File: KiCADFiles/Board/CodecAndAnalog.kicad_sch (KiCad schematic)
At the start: 38 parts, among them J1 XLR, J2 MONO JACK, J4 MONO JACK, J5 MONO JACK, J6 MONO JACK, J7 MONO JACK, K2 Fujitsu_FTR-LYCA005x, U5 CS4272, U9 OPA1655D, X1 24.576 MHz 20 pF

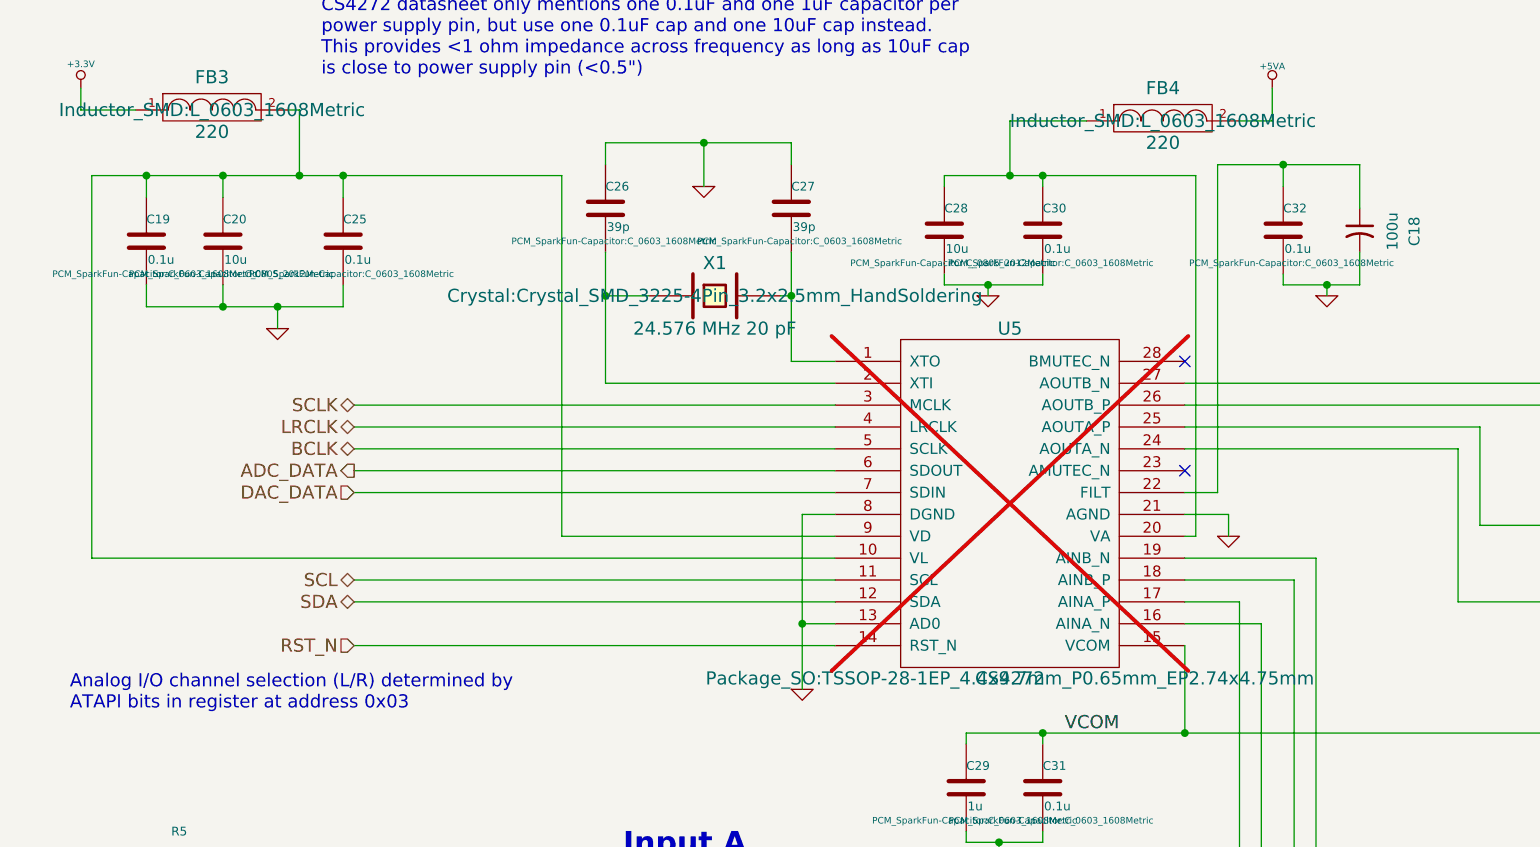
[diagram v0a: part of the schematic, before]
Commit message: improved layout further
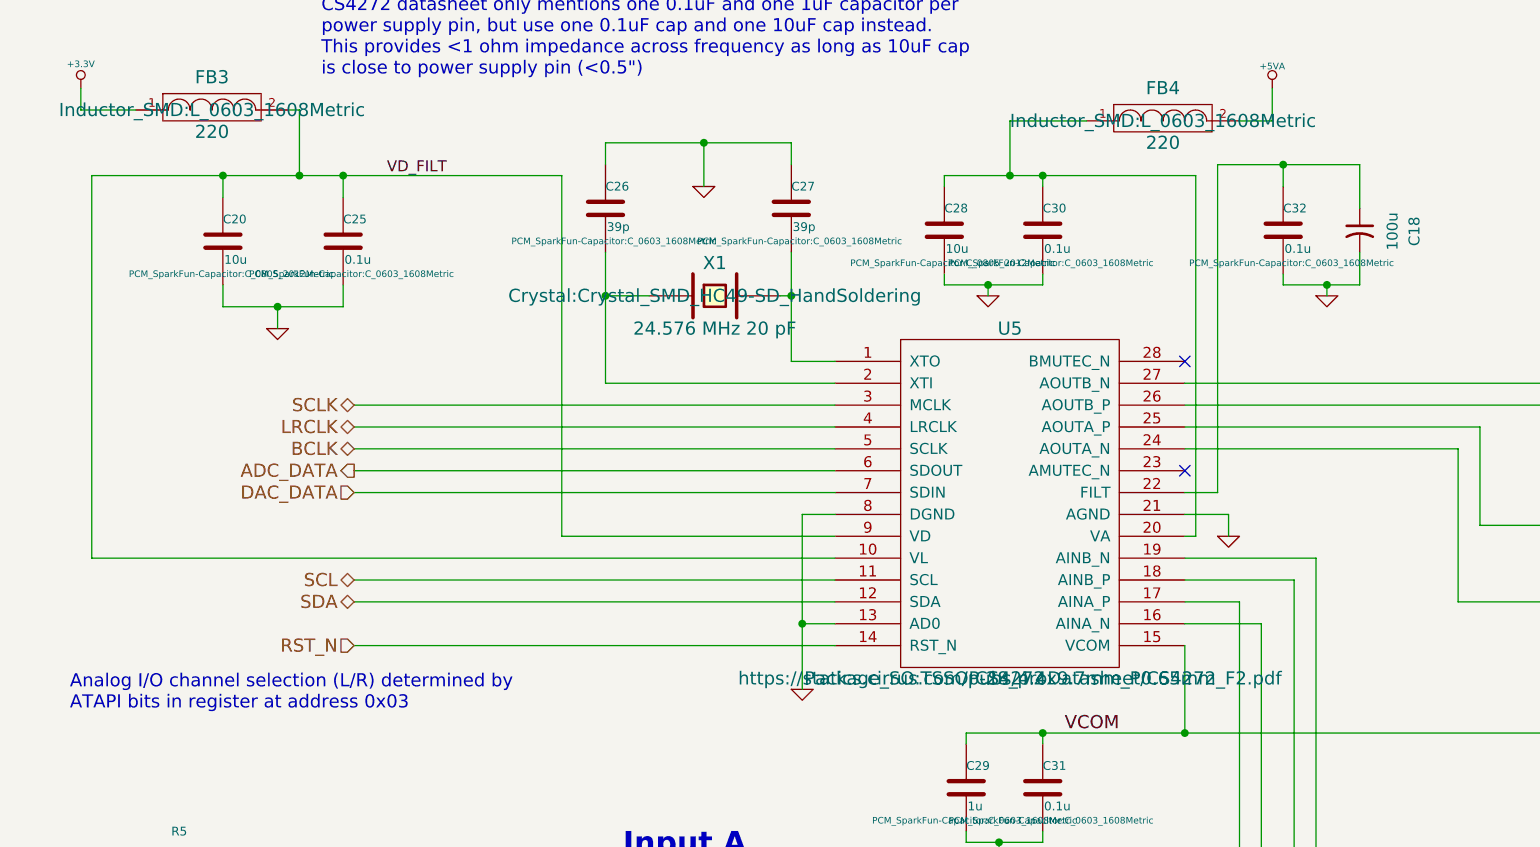
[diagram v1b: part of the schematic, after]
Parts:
- removed C19: 0.1u, PCM_SparkFun-Capacitor:C_0603_1608Metric, symbol SuperAudioBoard-rescue:C
- U5: footprint Package_SO:TSSOP-28-1EP_4.4x9.7mm_P0.65mm_EP2.74x4.75mm -> Package_SO:TSSOP-28_4.4x9.7mm_P0.65mm; now fitted
- X1: footprint Crystal:Crystal_SMD_3225-4Pin_3.2x2.5mm_HandSoldering -> Crystal:Crystal_SMD_HC49-SD_HandSoldering
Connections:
- net VD_FILT: now reaches C20.1, C25.1, FB3.2, U5.10 (VL), U5.9 (VD)
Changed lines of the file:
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@@
 	)
 	(junction
-		(at 25.4 29.21)
-		(diameter 0)
-		(color 0 0 0 0)
-	)
-	(junction
 		(at 129.54 93.98)
 		(diameter 0)
@@
 	)
 	(junction
-		(at 34.29 44.45)
-		(diameter 0)
-		(color 0 0 0 0)
-	)
-	(junction
 		(at 195.58 140.97)
 		(diameter 0)
@@
 	(wire
 		(pts
-			(xy 25.4 44.45) (xy 25.4 41.91)
-		)
-		(stroke
-			(width 0)
-			(type default)
-		)
-	)
-	(wire
-		(pts
 			(xy 134.62 22.86) (xy 125.73 22.86)
 		)
@@
 	(wire
 		(pts
-			(xy 25.4 44.45) (xy 34.29 44.45)
-		)
-		(stroke
-			(width 0)
-			(type default)
-		)
-	)
-	(wire
-		(pts
 			(xy 133.35 168.91) (xy 158.75 168.91)
 		)
@@
 	(wire
 		(pts
-			(xy 25.4 29.21) (xy 19.05 29.21)
+			(xy 19.05 29.21) (xy 34.29 29.21)
 		)
 		(stroke
@@
 	(wire
 		(pts
-			(xy 34.29 29.21) (xy 25.4 29.21)
-		)
-		(stroke
-			(width 0)
-			(type default)
-		)
-	)
-	(wire
-		(pts
 			(xy 49.53 58.42) (xy 105.41 58.42)
 		)
@@
 	(wire
 		(pts
-			(xy 25.4 29.21) (xy 25.4 31.75)
-		)
-		(stroke
-			(width 0)
-			(type default)
-		)
-	)
-	(wire
-		(pts
 			(xy 133.35 172.72) (xy 161.29 172.72)
 		)
@@
 		)
 	)
+	(label "VD_FILT"
+		(at 53.34 29.21 0)
+		(effects
+			(font
+				(size 1.27 1.27)
+			)
+			(justify left bottom)
+		)
+	)
 	(label "VCOM"
 		(at 138.43 93.98 180)
@@
 		(in_bom yes)
 		(on_board yes)
-		(dnp yes)
+		(dnp no)
 		(property "Reference" "U5"
 			(at 125.73 46.99 0)
@@
 			)
 		)
-		(property "Footprint" "Package_SO:TSSOP-28-1EP_4.4x9.7mm_P0.65mm_EP2.74x4.75mm"
+		(property "Footprint" "Package_SO:TSSOP-28_4.4x9.7mm_P0.65mm"
 			(at 125.73 87.63 0)
 			(effects
@@
 			)
 		)
-		(property "Datasheet" "~"
+		(property "Datasheet" "https://statics.cirrus.com/pubs/proDatasheet/CS4272_F2.pdf"
 			(at 125.73 87.63 0)
 			(effects
@@
 			)
 		)
-		(property "Footprint" "Crystal:Crystal_SMD_3225-4Pin_3.2x2.5mm_HandSoldering"
+		(property "Footprint" "Crystal:Crystal_SMD_HC49-SD_HandSoldering"
 			(at 91.44 43.18 0)
 			(effects
@@
 					(unit 1)
 				)
-			)
-		)
-	)
-	(symbol
-		(lib_name "C_19")
-		(lib_id "SuperAudioBoard-rescue:C")
-		(at 25.4 36.83 0)
-		(unit 1)
-		(exclude_from_sim no)
-		(in_bom yes)
-		(on_board yes)
-		(dnp no)
-		(property "Reference" "C19"
-			(at 25.4 34.29 0)
-			(effects
-				(font
-					(size 1.016 1.016)
-				)
-				(justify left)
-			)
-		)
-		(property "Value" "0.1u"
-			(at 25.5524 38.989 0)
-			(effects
-				(font
-					(size 1.016 1.016)
-				)
-				(justify left)
-			)
-		)
-		(property "Footprint" "PCM_SparkFun-Capacitor:C_0603_1608Metric"
-			(at 26.3652 40.64 0)
-			(effects
-				(font
-					(size 0.762 0.762)
-				)
-			)
-		)
-		(property "Datasheet" "~"
-			(at 25.4 36.83 0)
-			(effects
-				(font
-					(size 1.524 1.524)
-				)
-			)
-		)
-		(property "Description" ""
-			(at 25.4 36.83 0)
-			(effects
-				(font
-					(size 1.27 1.27)
-				)
-			)
-		)
-		(property "MFG 1 Name" "Murata"
-			(at 25.4 36.83 0)
-			(effects
-				(font
-					(size 1.524 1.524)
-				)
-				(hide yes)
-			)
-		)
-		(property "MFG1 PN" "GRM188R71E104KA01"
-			(at 25.4 36.83 0)
-			(effects
-				(font
-					(size 1.524 1.524)
-				)
-				(hide yes)
-			)
-		)
-		(property "MFG 2 Name" "TDK"
-			(at 25.4 36.83 0)
-			(effects
-				(font
-					(size 1.524 1.524)
-				)
-				(hide yes)
-			)
-		)
-		(property "MFG 2 PN" "C1608X7R1E104K080AA"
-			(at 25.4 36.83 0)
-			(effects
-				(font
-					(size 1.524 1.524)
-				)
-				(hide yes)
-			)
-		)
-		(property "MPN" "CL10B104KB8NNNL"
-			(at 25.4 36.83 0)
-			(effects
-				(font
-					(size 1.27 1.27)
-				)
-				(hide yes)
-			)
-		)
-		(property "Tol" ""
-			(at 25.4 36.83 0)
-			(effects
-				(font
-					(size 1.27 1.27)
-				)
-				(hide yes)
-			)
-		)
-		(pin "1"
-		)
-		(pin "2"
-		)
-		(instances
-			(project "SuperAudioBoard"
-				(path "/01f65e03-4e05-4001-87b4-b3e88e4198ab/00000000-0000-0000-0000-00005438c479"
-					(reference "C19")
-					(unit 1)
-				)
